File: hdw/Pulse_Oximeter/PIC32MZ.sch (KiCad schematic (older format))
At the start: 1 part

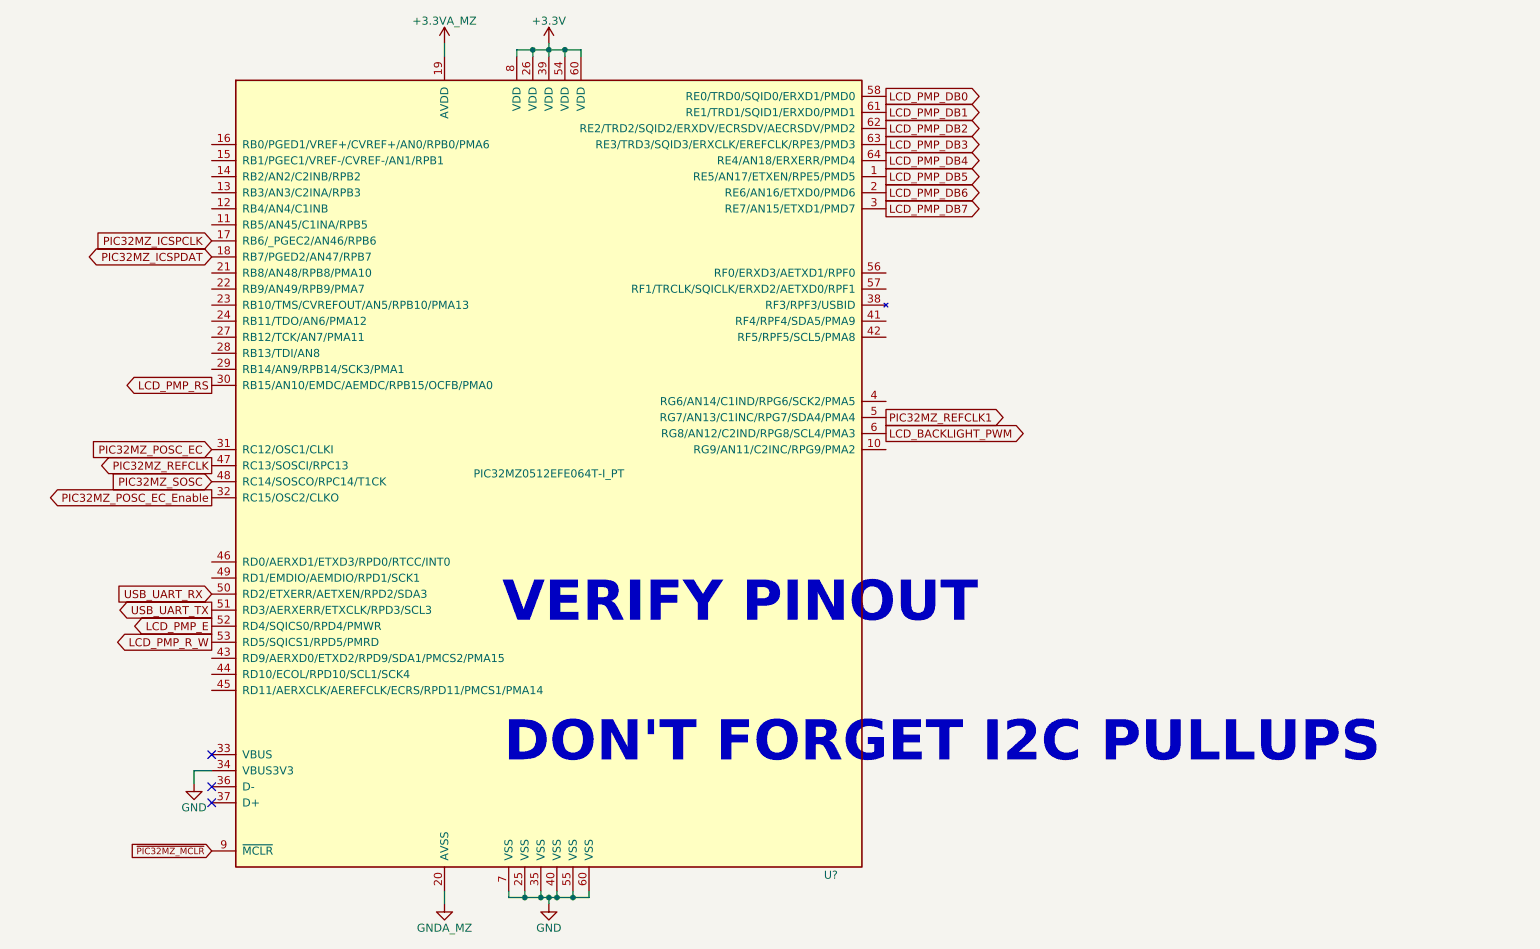
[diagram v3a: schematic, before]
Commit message: Added I2C to PIC32MZ
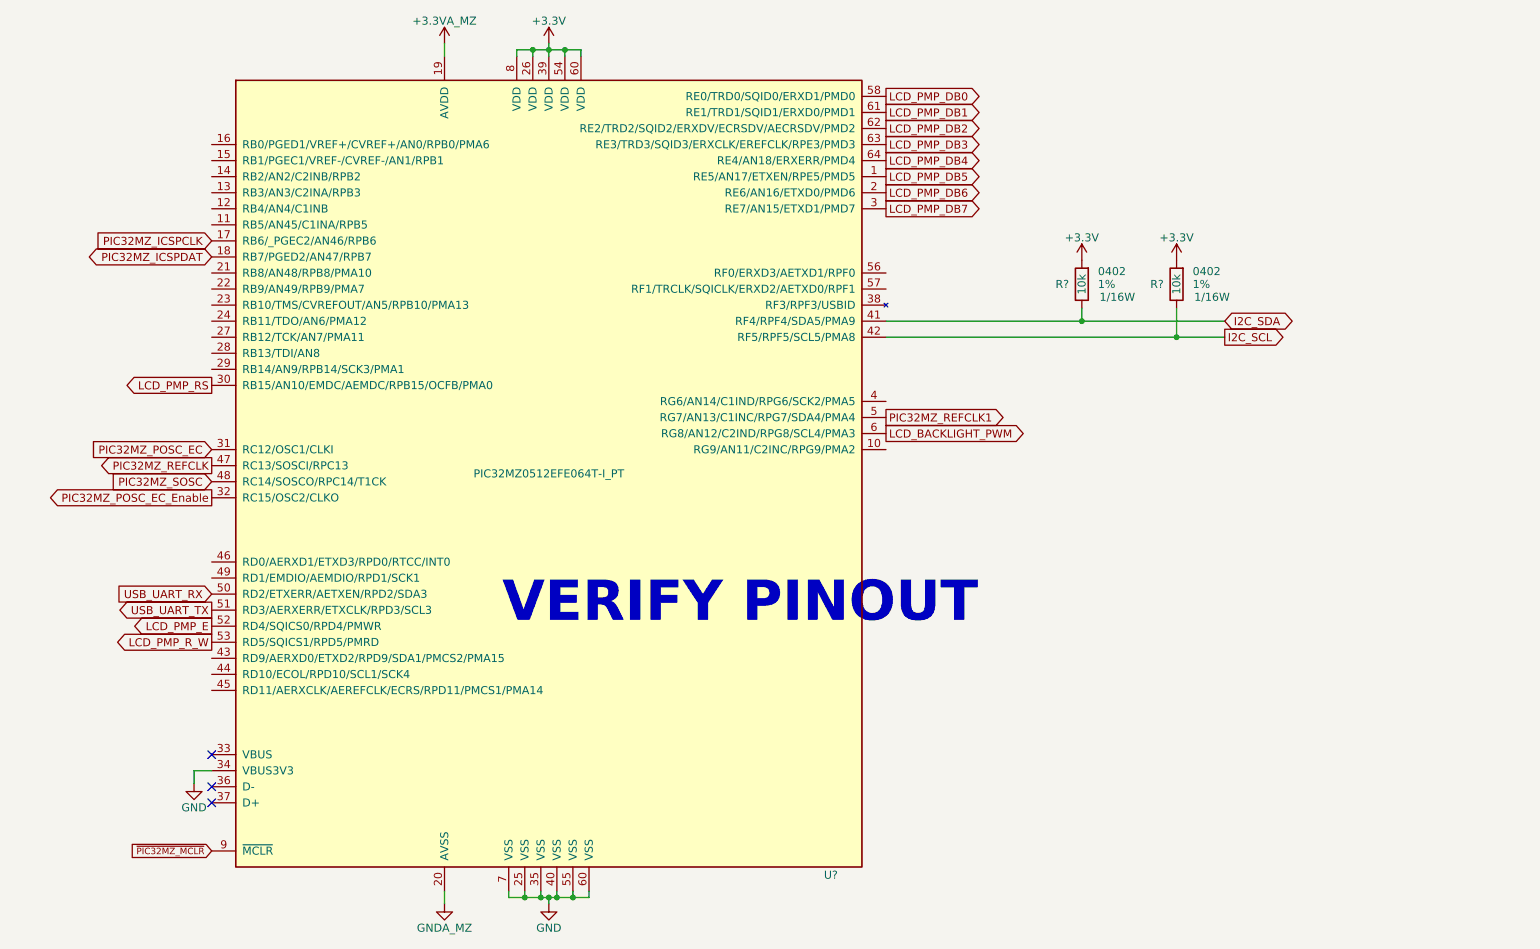
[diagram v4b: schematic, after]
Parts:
- added R? (x2): 10k, Resistors_SMD:R_0402, symbol Custom_Library:R_Custom
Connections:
- net +3V3: now also R?.1, R?.1
- net I2C_SDA: now reaches U?.41 (RF4/RPF4/SDA5/PMA9)
- net I2C_SDA: now also R?.2
- net I2C_SCL: now reaches U?.42 (RF5/RPF5/SCL5/PMA8)
- net I2C_SCL: now also R?.2
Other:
- note removed: "DON'T FORGET I2C PULLUPS"
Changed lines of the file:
@@
 Text GLabel 7560 3210 2    50   Output ~ 0
 PIC32MZ_REFCLK1
-Text Notes 5180 5380 0    250  ~ 50
-DON'T FORGET I2C PULLUPS
+Text GLabel 9670 2710 2    50   Output ~ 0
+I2C_SCL
+Text GLabel 9670 2610 2    50   BiDi ~ 0
+I2C_SDA
+Wire Wire Line
+	7560 2610 8780 2610
+Wire Wire Line
+	7560 2710 9370 2710
+$Comp
+L Custom_Library:R_Custom R?
+U 1 1 5EB7DAD1
+P 9370 2380
+AR Path="/5BB27BA3/5EB7DAD1" Ref="R?"  Part="1"
+AR Path="/5BB27BF7/5EB7DAD1" Ref="R?"  Part="1"
+AR Path="/5C1DE17A/5EB7DAD1" Ref="R?"  Part="1"
+AR Path="/5C1E3A08/5EB7DAD1" Ref="R?"  Part="1"
+AR Path="/5D779AE1/5EB7DAD1" Ref="R?"  Part="1"
+AR Path="/5CB7718D/5EB7DAD1" Ref="R?"  Part="1"
+AR Path="/5E0DC082/5EB7DAD1" Ref="R?"  Part="1"
+AR Path="/5E0F9110/5EB7DAD1" Ref="R?"  Part="1"
+AR Path="/5E9E0EA5/5EB7DAD1" Ref="R?"  Part="1"
+AR Path="/5E9E0E87/5EB7DAD1" Ref="R?"  Part="1"
+AR Path="/5EAE2D66/5EB7DAD1" Ref="R?"  Part="1"
+AR Path="/5EAE4A89/5EB7DAD1" Ref="R?"  Part="1"
+F 0 "R?" H 9290 2380 50  0000 R CNN
+F 1 "10k" V 9370 2380 50  0000 C CNN
+F 2 "Resistors_SMD:R_0402" H 9370 2380 50  0001 C CNN
+F 3 "" H 9370 2380 50  0001 C CNN
+F 4 "0402" H 9470 2460 50  0000 L CNN "display_footprint"
+F 5 "1%" H 9470 2380 50  0000 L CNN "Tolerance"
+F 6 "1/16W" H 9480 2300 50  0000 L CNN "Wattage"
+	1    9370 2380
+	1    0    0    -1
+$EndComp
+$Comp
+L power:+3.3V #PWR?
+U 1 1 5EB7DAD7
+P 9370 2230
+F 0 "#PWR?" H 9370 2080 50  0001 C CNN
+F 1 "+3.3V" H 9370 2370 50  0000 C CNN
+F 2 "" H 9370 2230 50  0001 C CNN
+F 3 "" H 9370 2230 50  0001 C CNN
+	1    9370 2230
+	1    0    0    -1
+$EndComp
+$Comp
+L Custom_Library:R_Custom R?
+U 1 1 5EB7DEAB
+P 8780 2380
+AR Path="/5BB27BA3/5EB7DEAB" Ref="R?"  Part="1"
+AR Path="/5BB27BF7/5EB7DEAB" Ref="R?"  Part="1"
+AR Path="/5C1DE17A/5EB7DEAB" Ref="R?"  Part="1"
+AR Path="/5C1E3A08/5EB7DEAB" Ref="R?"  Part="1"
+AR Path="/5D779AE1/5EB7DEAB" Ref="R?"  Part="1"
+AR Path="/5CB7718D/5EB7DEAB" Ref="R?"  Part="1"
+AR Path="/5E0DC082/5EB7DEAB" Ref="R?"  Part="1"
+AR Path="/5E0F9110/5EB7DEAB" Ref="R?"  Part="1"
+AR Path="/5E9E0EA5/5EB7DEAB" Ref="R?"  Part="1"
+AR Path="/5E9E0E87/5EB7DEAB" Ref="R?"  Part="1"
+AR Path="/5EAE2D66/5EB7DEAB" Ref="R?"  Part="1"
+AR Path="/5EAE4A89/5EB7DEAB" Ref="R?"  Part="1"
+F 0 "R?" H 8700 2380 50  0000 R CNN
+F 1 "10k" V 8780 2380 50  0000 C CNN
+F 2 "Resistors_SMD:R_0402" H 8780 2380 50  0001 C CNN
+F 3 "" H 8780 2380 50  0001 C CNN
+F 4 "0402" H 8880 2460 50  0000 L CNN "display_footprint"
+F 5 "1%" H 8880 2380 50  0000 L CNN "Tolerance"
+F 6 "1/16W" H 8890 2300 50  0000 L CNN "Wattage"
+	1    8780 2380
+	1    0    0    -1
+$EndComp
+$Comp
+L power:+3.3V #PWR?
+U 1 1 5EB7DEB5
+P 8780 2230
+F 0 "#PWR?" H 8780 2080 50  0001 C CNN
+F 1 "+3.3V" H 8780 2370 50  0000 C CNN
+F 2 "" H 8780 2230 50  0001 C CNN
+F 3 "" H 8780 2230 50  0001 C CNN
+	1    8780 2230
+	1    0    0    -1
+$EndComp
+Wire Wire Line
+	8780 2530 8780 2610
+Connection ~ 8780 2610
+Wire Wire Line
+	8780 2610 9670 2610
+Wire Wire Line
+	9370 2530 9370 2710
+Connection ~ 9370 2710
+Wire Wire Line
+	9370 2710 9670 2710
 $EndSCHEMATC
